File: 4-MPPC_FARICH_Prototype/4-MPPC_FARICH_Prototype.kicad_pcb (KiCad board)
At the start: 8 copper layers, 164.2 x 53.4 mm, 17 parts, among them J1 1778764, J10 ST4-40-1.00-L-D-P-TR, J11 ST4-40-1.00-L-D-P-TR, J12 ST4-40-1.00-L-D-P-TR, J13 ST4-40-1.00-L-D-P-TR, J2 ST4-40-1.00-L-D-P-TR, J3 ST4-40-1.00-L-D-P-TR, J4 ST4-40-1.00-L-D-P-TR, J5 ST4-40-1.00-L-D-P-TR, J6 ST4-40-1.00-L-D-P-TR, J7 ST4-40-1.00-L-D-P-TR, J8 ST4-40-1.00-L-D-P-TR, J9 ST4-40-1.00-L-D-P-TR

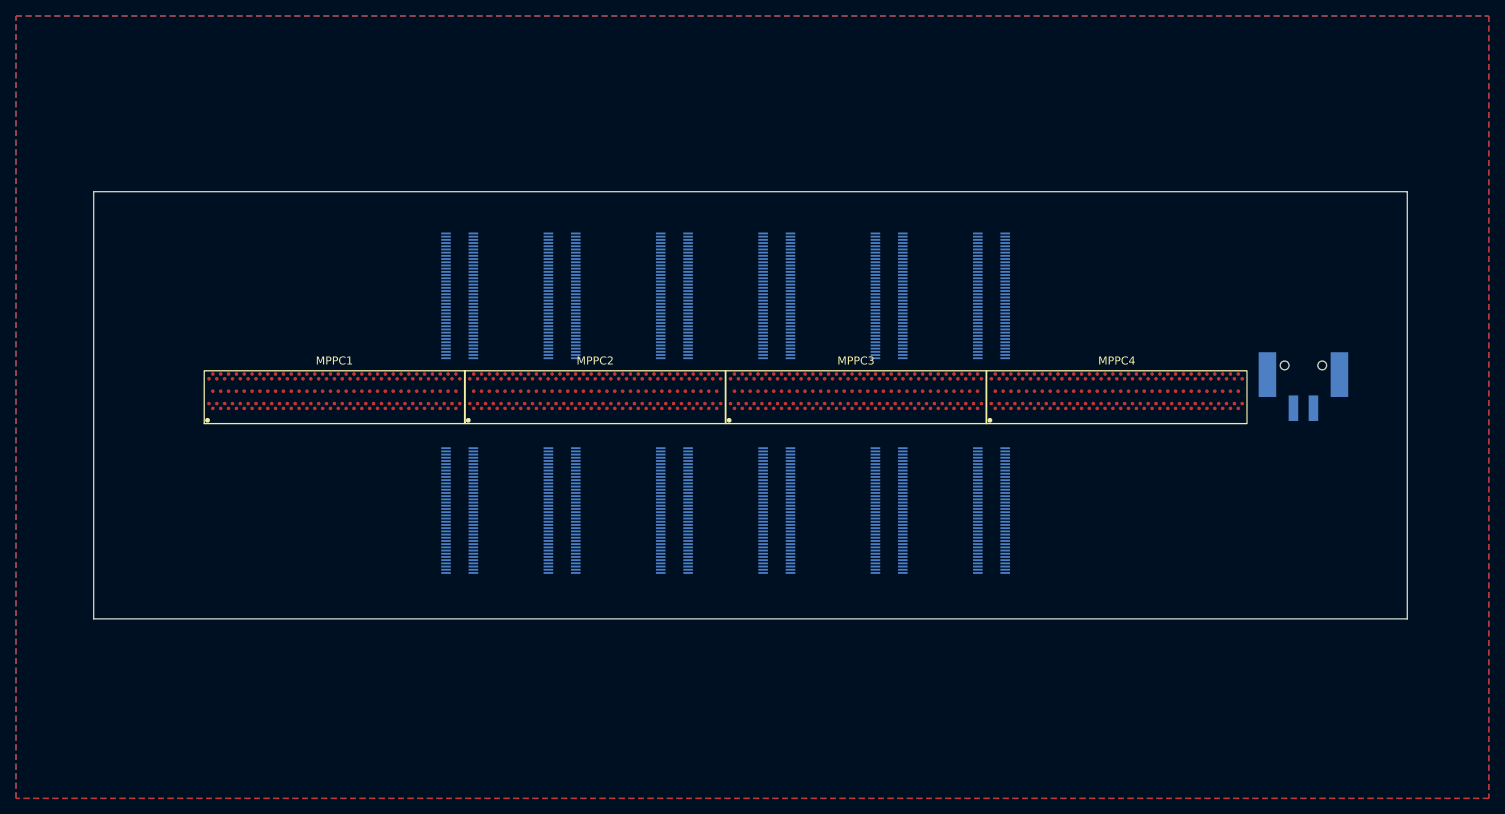
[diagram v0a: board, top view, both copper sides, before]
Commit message: .
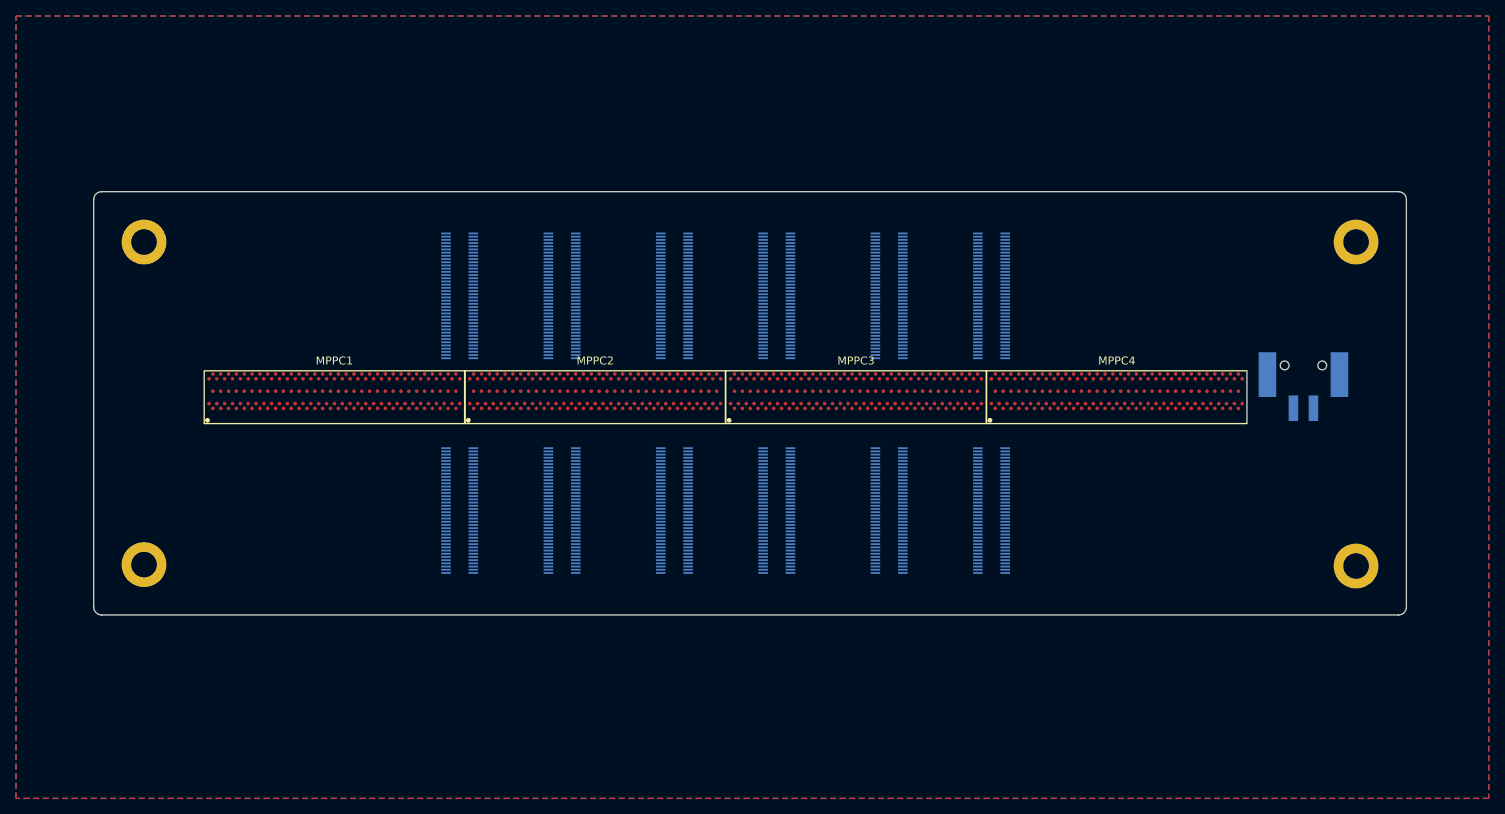
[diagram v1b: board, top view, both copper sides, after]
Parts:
- added H1: MountingHole, MountingHole:MountingHole_3.2mm_M3_DIN965_Pad, F.Cu at (73.2, 72.4)
- added H2: MountingHole, MountingHole:MountingHole_3.2mm_M3_DIN965_Pad, F.Cu at (73.2, 112.7)
- added H3: MountingHole, MountingHole:MountingHole_3.2mm_M3_DIN965_Pad, F.Cu at (224.7, 72.4)
- added H4: MountingHole, MountingHole:MountingHole_3.2mm_M3_DIN965_Pad, F.Cu at (224.7, 112.9)
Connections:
- J1 pad SH1: GND -> (no net)
- J1 pad SH2: GND -> (no net)
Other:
- board size 164.2 x 53.4 mm -> 164.1 x 52.9 mm
